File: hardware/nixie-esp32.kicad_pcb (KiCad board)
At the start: 6 copper layers, 66 x 74 mm, 56 parts, among them IC1 MCP1661T-E_OT, IC2 CD4504BM, J1 USB4216-03-A_REVA, SW1 RESET, SW2 BOOT, U1 AP7361C-33E-13, U2 ESP32-S3-WROOM-1, U3 SN74AHCT1G125DBVR, U4 HV5622PG

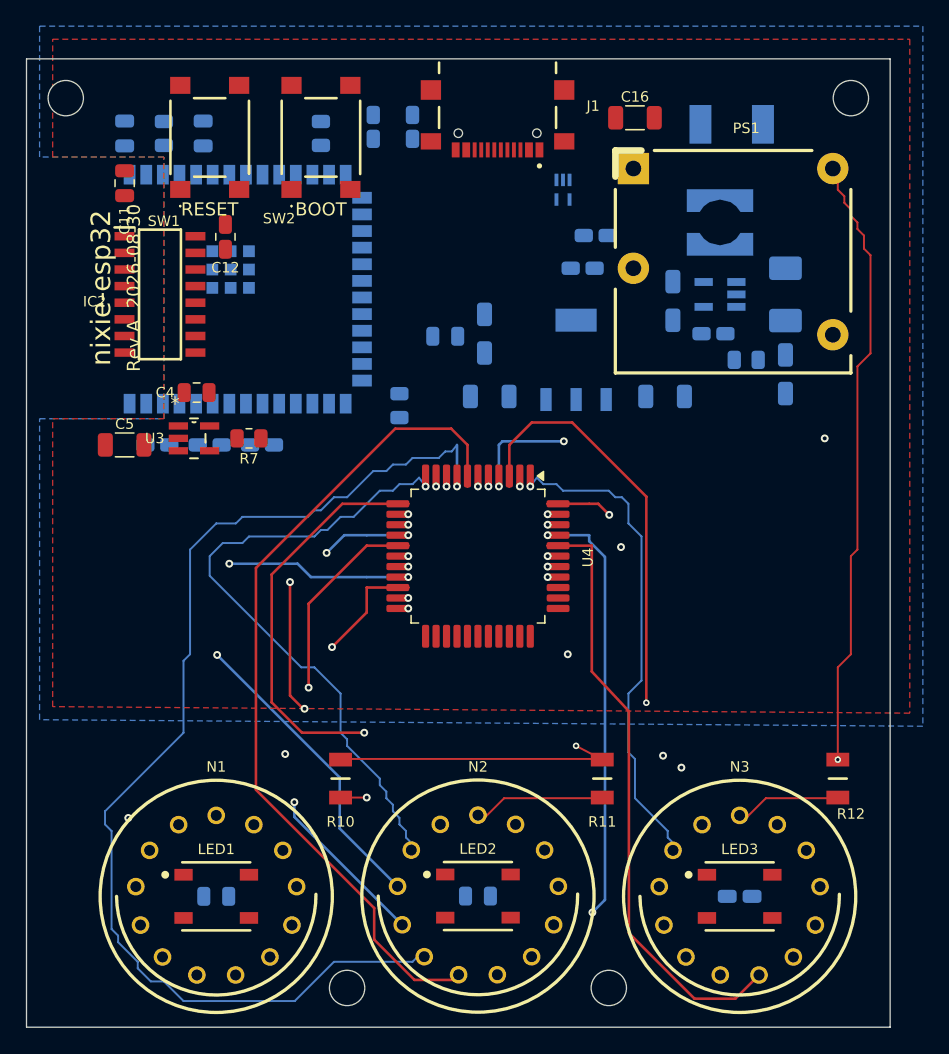
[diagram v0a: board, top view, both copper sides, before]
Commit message: WIP SN74141 redesign
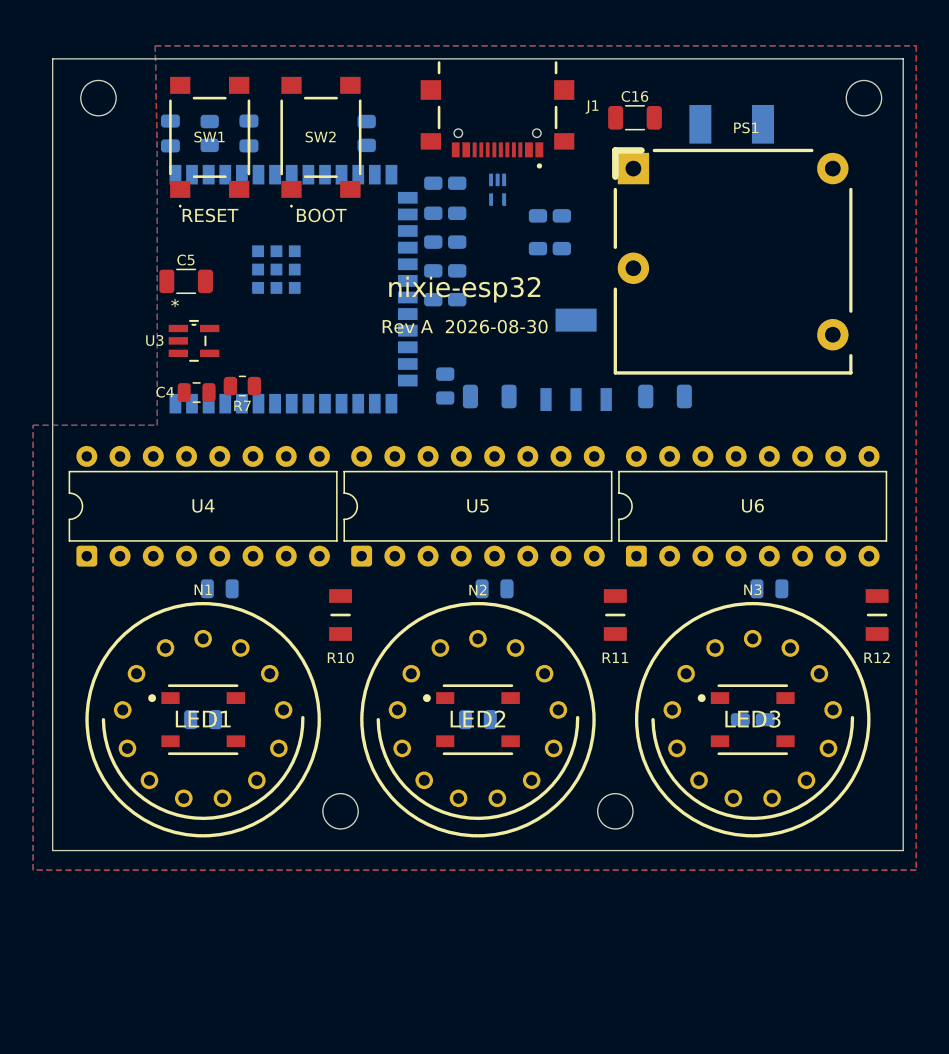
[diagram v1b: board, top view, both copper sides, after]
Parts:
- removed C10, C14, C9: 10µF, Capacitor_SMD:C_1206_3216Metric
- removed D5: SS14-HF, Diode_SMD:D_SMA
- removed IC1: MCP1661T-E_OT, nixie-esp32:SOT95P270X145-5N
- removed IC2: CD4504BM, nixie-esp32:SOIC127P600X175-16N
- removed L1: 4.7µH, nixie-esp32:MSS5131
- removed R8: 1.05M, Resistor_SMD:R_0805_2012Metric
- removed R9: 120k, Resistor_SMD:R_0805_2012Metric
- added U5: SN74141N, Package_DIP:DIP-16_W7.62mm, F.Cu at (142.6, 114.5)
- added U6: SN74141N, Package_DIP:DIP-16_W7.62mm, F.Cu at (163.6, 114.5)
- C11, C12: moved to B.Cu
- U4: value HV5622PG -> SN74141N; footprint Package_QFP:PQFP-44_10x10mm_P0.8mm -> Package_DIP:DIP-16_W7.62mm
- moved C12 33.9 mm to (152.8, 117.0), turned to 180 degrees
- moved C11 31.8 mm to (131.8, 117.0), turned to 180 degrees
- moved C13 31.4 mm to (173.8, 117.0), turned to 180 degrees
- moved U4 29.9 mm to (121.6, 114.5), turned to 90 degrees
- moved R15 26.9 mm to (149.0, 90.5)
- moved R16 22.4 mm to (149.0, 92.7)
- moved R13 17.9 mm to (149.0, 94.9)
- moved C6 13.5 mm to (130.5, 127.0)
- moved C8 13.5 mm to (172.5, 127.0)
- moved LED1 13.5 mm to (130.5, 127.0)
- moved LED3 13.5 mm to (172.5, 127.0)
- moved N1 13.5 mm to (130.5, 127.0)
- moved N3 13.5 mm to (172.5, 127.0)
- moved H3 13.5 mm to (141.0, 134.0)
- moved H4 13.5 mm to (162.0, 134.0)
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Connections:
- C12 pad 1: +12V -> +5V
- C13 pad 1: GND -> +5V
- C13 pad 2: +12V -> GND
- N1 pad 0: /Nixies/HvDriver/Nixie1/K0 -> /Nixies/HvDriver/N1_K0
- N1 pad 1: /Nixies/HvDriver/Nixie1/K1 -> /Nixies/HvDriver/N1_K1
- N1 pad 2: /Nixies/HvDriver/Nixie1/K2 -> /Nixies/HvDriver/N1_K2
- N1 pad 3: /Nixies/HvDriver/Nixie1/K3 -> /Nixies/HvDriver/N1_K3
- N1 pad 4: /Nixies/HvDriver/Nixie1/K4 -> /Nixies/HvDriver/N1_K4
- N1 pad 5: /Nixies/HvDriver/Nixie1/K5 -> /Nixies/HvDriver/N1_K5
- N1 pad 6: /Nixies/HvDriver/Nixie1/K6 -> /Nixies/HvDriver/N1_K6
- N1 pad 7: /Nixies/HvDriver/Nixie1/K7 -> /Nixies/HvDriver/N1_K7
- N1 pad 8: /Nixies/HvDriver/Nixie1/K8 -> /Nixies/HvDriver/N1_K8
- N1 pad 9: /Nixies/HvDriver/Nixie1/K9 -> /Nixies/HvDriver/N1_K9
- N2 pad 0: /Nixies/HvDriver/Nixie2/K0 -> /Nixies/HvDriver/N2_K0
- N2 pad 1: /Nixies/HvDriver/Nixie2/K1 -> /Nixies/HvDriver/N2_K1
- N2 pad 2: /Nixies/HvDriver/Nixie2/K2 -> /Nixies/HvDriver/N2_K2
- N2 pad 3: /Nixies/HvDriver/Nixie2/K3 -> /Nixies/HvDriver/N2_K3
- N2 pad 4: /Nixies/HvDriver/Nixie2/K4 -> /Nixies/HvDriver/N2_K4
- N2 pad 5: /Nixies/HvDriver/Nixie2/K5 -> /Nixies/HvDriver/N2_K5
- N2 pad 6: /Nixies/HvDriver/Nixie2/K6 -> /Nixies/HvDriver/N2_K6
- N2 pad 7: /Nixies/HvDriver/Nixie2/K7 -> /Nixies/HvDriver/N2_K7
- N2 pad 8: /Nixies/HvDriver/Nixie2/K8 -> /Nixies/HvDriver/N2_K8
- N2 pad 9: /Nixies/HvDriver/Nixie2/K9 -> /Nixies/HvDriver/N2_K9
- N3 pad 0: /Nixies/HvDriver/Nixie3/K0 -> /Nixies/HvDriver/N3_K0
- N3 pad 1: /Nixies/HvDriver/Nixie3/K1 -> /Nixies/HvDriver/N3_K1
- N3 pad 2: /Nixies/HvDriver/Nixie3/K2 -> /Nixies/HvDriver/N3_K2
- N3 pad 3: /Nixies/HvDriver/Nixie3/K3 -> /Nixies/HvDriver/N3_K3
- N3 pad 4: /Nixies/HvDriver/Nixie3/K4 -> /Nixies/HvDriver/N3_K4
- N3 pad 5: /Nixies/HvDriver/Nixie3/K5 -> /Nixies/HvDriver/N3_K5
- N3 pad 6: /Nixies/HvDriver/Nixie3/K6 -> /Nixies/HvDriver/N3_K6
- N3 pad 7: /Nixies/HvDriver/Nixie3/K7 -> /Nixies/HvDriver/N3_K7
- N3 pad 8: /Nixies/HvDriver/Nixie3/K8 -> /Nixies/HvDriver/N3_K8
- N3 pad 9: /Nixies/HvDriver/Nixie3/K9 -> /Nixies/HvDriver/N3_K9
- U2 pad 10: unconnected-(U2-GPIO17/U1TXD/ADC2_CH6-Pad10) -> ESP32_GPIO17
- U2 pad 11: unconnected-(U2-GPIO18/U1RXD/ADC2_CH7/CLK_OUT3-Pad11) -> ESP32_GPIO18
- U2 pad 20: unconnected-(U2-GPIO12/TOUCH12/ADC2_CH1/FSPICLK/FSPIIO6/SUBSPICLK-Pad20) -> ESP32_GPIO12
- U2 pad 21: unconnected-(U2-GPIO13/TOUCH13/ADC2_CH2/FSPIQ/FSPIIO7/SUBSPIQ-Pad21) -> ESP32_GPIO13
- U2 pad 22: unconnected-(U2-GPIO14/TOUCH14/ADC2_CH3/FSPIWP/FSPIDQS/SUBSPIWP-Pad22) -> ESP32_GPIO14
- U2 pad 23: unconnected-(U2-GPIO21-Pad23) -> ESP32_GPIO21
- U2 pad 31: unconnected-(U2-GPIO38/FSPIWP/SUBSPIWP-Pad31) -> ESP32_GPIO38
- U2 pad 38: unconnected-(U2-GPIO2/TOUCH2/ADC1_CH1-Pad38) -> ESP32_GPIO2
- U2 pad 39: unconnected-(U2-GPIO1/TOUCH1/ADC1_CH0-Pad39) -> ESP32_GPIO1
- U2 pad 5: unconnected-(U2-GPIO5/TOUCH5/ADC1_CH4-Pad5) -> ESP32_GPIO5
- U2 pad 6: unconnected-(U2-GPIO6/TOUCH6/ADC1_CH5-Pad6) -> ESP32_GPIO6
- U2 pad 7: unconnected-(U2-GPIO7/TOUCH7/ADC1_CH6-Pad7) -> ESP32_GPIO7
- U4 pad 1: /Nixies/HvDriver/Nixie3/K1 -> /Nixies/HvDriver/N1_K8
- U4 pad 10: /Nixies/HvDriver/Nixie2/K2 -> /Nixies/HvDriver/N1_K7
- U4 pad 11: /Nixies/HvDriver/Nixie2/K1 -> /Nixies/HvDriver/N1_K6
- U4 pad 12: /Nixies/HvDriver/Nixie2/K0 -> GND
- U4 pad 13: /Nixies/HvDriver/Nixie1/K9 -> /Nixies/HvDriver/N1_K4
- U4 pad 14: /Nixies/HvDriver/Nixie1/K8 -> /Nixies/HvDriver/N1_K5
- U4 pad 15: /Nixies/HvDriver/Nixie1/K7 -> /Nixies/HvDriver/N1_K0
- U4 pad 16: /Nixies/HvDriver/Nixie1/K6 -> /Nixies/HvDriver/N1_K2
- U4 pad 2: /Nixies/HvDriver/Nixie3/K0 -> /Nixies/HvDriver/N1_K9
- U4 pad 3: /Nixies/HvDriver/Nixie2/K9 -> ESP32_GPIO1
- U4 pad 4: /Nixies/HvDriver/Nixie2/K8 -> ESP32_GPIO6
- U4 pad 5: /Nixies/HvDriver/Nixie2/K7 -> +5V
- U4 pad 6: /Nixies/HvDriver/Nixie2/K6 -> ESP32_GPIO2
- U4 pad 7: /Nixies/HvDriver/Nixie2/K5 -> ESP32_GPIO5
- U4 pad 8: /Nixies/HvDriver/Nixie2/K4 -> /Nixies/HvDriver/N1_K1
- U4 pad 9: /Nixies/HvDriver/Nixie2/K3 -> /Nixies/HvDriver/N1_K3
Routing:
- net /Nixies/HvDriver/Nixie2/K6: track 98.8 -> 0.00 mm, vias 1 -> 0
- net +170V: track 90.8 -> 0.00 mm, vias 2 -> 0
- net /Nixies/HvDriver/Nixie2/K4: track 87.8 -> 0.00 mm, vias 1 -> 0
- net /Nixies/HvDriver/Nixie2/K5: track 65.1 -> 0.00 mm
- net /Nixies/HvDriver/Nixie2/K7: track 61.9 -> 0.00 mm, vias 2 -> 0
- net /Nixies/HvDriver/Nixie3/K0: track 59.7 -> 0.00 mm, vias 2 -> 0
- net /Nixies/HvDriver/Nixie3/K9: track 53.0 -> 0.00 mm, vias 1 -> 0
- net /Nixies/HvDriver/Nixie2/K8: track 52.7 -> 0.00 mm, vias 3 -> 0
- net /Nixies/HvDriver/Nixie2/K3: track 52.7 -> 0.00 mm, vias 2 -> 0
- net /Nixies/HvDriver/Nixie2/K2: track 51.9 -> 0.00 mm, vias 2 -> 0
- net /Nixies/HvDriver/Nixie1/K5: track 51.8 -> 0.00 mm, vias 1 -> 0
- net /Nixies/HvDriver/Nixie2/K0: track 50.1 -> 0.00 mm, vias 1 -> 0
- net /Nixies/HvDriver/Nixie2/K9: track 50.1 -> 0.00 mm, vias 1 -> 0
- net /Nixies/HvDriver/Nixie1/K4: track 50.0 -> 0.00 mm, vias 1 -> 0
- net /Nixies/HvDriver/Nixie2/K1: track 49.6 -> 0.00 mm, vias 1 -> 0
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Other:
- board size 66 x 74 mm -> 65 x 60.5 mm
- copper layers 6 -> 2
